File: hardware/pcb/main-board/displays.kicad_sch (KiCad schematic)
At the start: 1 part, among them J601 DISP_PCB x40 FPC

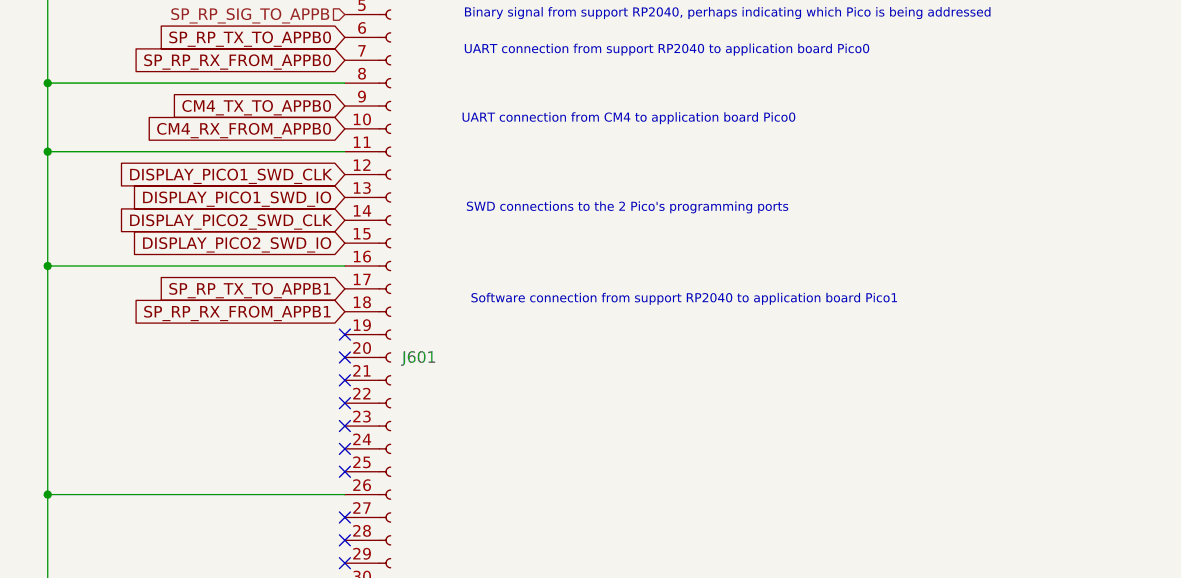
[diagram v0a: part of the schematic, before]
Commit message: tidy the keyboard comms
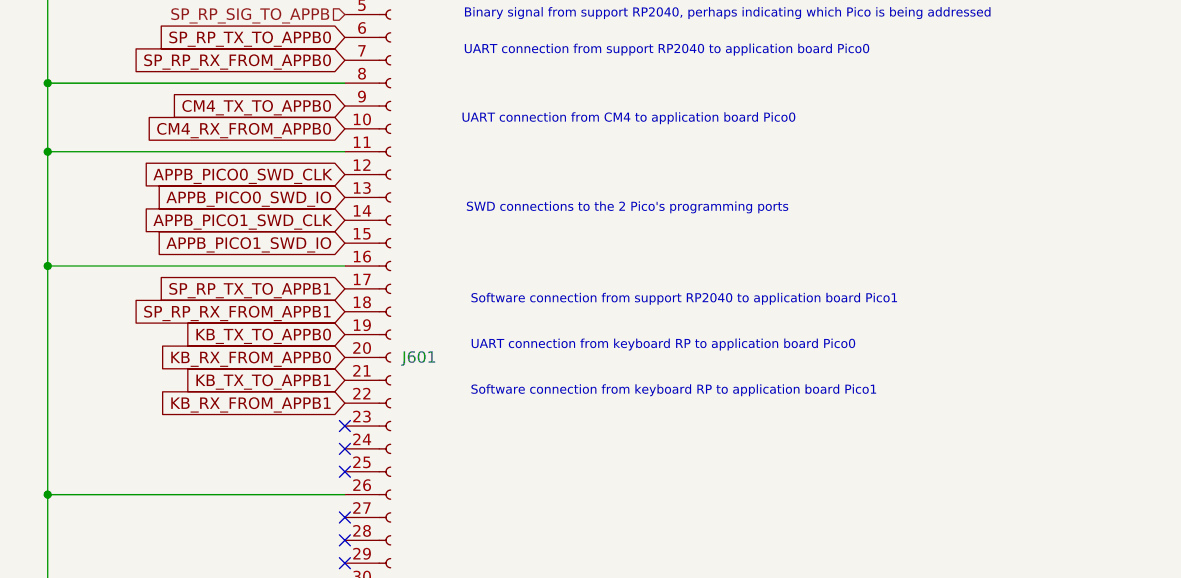
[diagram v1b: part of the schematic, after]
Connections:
- net KB_TX_TO_APPB0: now reaches J601.19 (Pin_19)
- net KB_RX_FROM_APPB0: now reaches J601.20 (Pin_20)
- net KB_TX_TO_APPB1: now reaches J601.21 (Pin_21)
- net KB_RX_FROM_APPB1: now reaches J601.22 (Pin_22)
- net DISPLAY_PICO1_SWD_CLK renamed APPB_PICO0_SWD_CLK
- net DISPLAY_PICO1_SWD_IO renamed APPB_PICO0_SWD_IO
- net DISPLAY_PICO2_SWD_CLK renamed APPB_PICO1_SWD_CLK
- net DISPLAY_PICO2_SWD_IO renamed APPB_PICO1_SWD_IO
- no-connect marks 15 -> 11
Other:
- note added: "Software connection from keyboard RP to application board Pico1"
- note added: "UART connection from keyboard RP to application board Pico0"
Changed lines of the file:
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@@
-	)
-	(no_connect
-		(at 58.42 68.58)
 	)
 	(no_connect
@@
 	)
 	(no_connect
-		(at 58.42 76.2)
-	)
-	(no_connect
-		(at 58.42 71.12)
-	)
-	(no_connect
 		(at 58.42 101.6)
 	)
@@
 		(at 58.42 99.06)
 	)
-	(no_connect
-		(at 58.42 73.66)
-	)
 	(wire
 		(pts
@@
 		)
 	)
+	(text "Software connection from keyboard RP to application board Pico1"
+		(exclude_from_sim no)
+		(at 72.39 74.93 0)
+		(effects
+			(font
+				(size 1 1)
+			)
+			(justify left)
+		)
+	)
 	(text "Software connection from support RP2040 to application board Pico1"
 		(exclude_from_sim no)
@@
 		)
 	)
+	(text "UART connection from keyboard RP to application board Pico0"
+		(exclude_from_sim no)
+		(at 72.39 69.85 0)
+		(effects
+			(font
+				(size 1 1)
+			)
+			(justify left)
+		)
+	)
 	(text "UART connection from CM4 to application board Pico0"
 		(exclude_from_sim no)
@@
 		)
 	)
-	(global_label "DISPLAY_PICO2_SWD_IO"
+	(global_label "APPB_PICO1_SWD_IO"
 		(shape input)
 		(at 58.42 58.42 180)
@@
 		)
 		(property "Intersheetrefs" "${INTERSHEET_REFS}"
-			(at 34.0756 58.42 0)
+			(at 36.7366 58.42 0)
 			(effects
 				(font
@@
 		)
 	)
-	(global_label "DISPLAY_PICO2_SWD_CLK"
+	(global_label "APPB_PICO1_SWD_CLK"
 		(shape input)
 		(at 58.42 55.88 180)
@@
 		)
 		(property "Intersheetrefs" "${INTERSHEET_REFS}"
-			(at 32.4428 55.88 0)
+			(at 35.1038 55.88 0)
 			(effects
 				(font
@@
 		)
 	)
-	(global_label "DISPLAY_PICO1_SWD_CLK"
+	(global_label "APPB_PICO0_SWD_CLK"
 		(shape input)
 		(at 58.42 50.8 180)
@@
 		)
 		(property "Intersheetrefs" "${INTERSHEET_REFS}"
-			(at 32.4428 50.8 0)
+			(at 35.1038 50.8 0)
 			(effects
 				(font
@@
 		)
 	)
-	(global_label "DISPLAY_PICO1_SWD_IO"
+	(global_label "KB_TX_TO_APPB1"
+		(shape input)
+		(at 58.42 73.66 180)
+		(fields_autoplaced yes)
+		(effects
+			(font
+				(size 1.27 1.27)
+			)
+			(justify right)
+		)
+		(property "Intersheetrefs" "${INTERSHEET_REFS}"
+			(at 40.0629 73.66 0)
+			(effects
+				(font
+					(size 1.27 1.27)
+				)
+				(justify right)
+				(hide yes)
+			)
+		)
+	)
+	(global_label "KB_RX_FROM_APPB0"
+		(shape input)
+		(at 58.42 71.12 180)
+		(fields_autoplaced yes)
+		(effects
+			(font
+				(size 1.27 1.27)
+			)
+			(justify right)
+		)
+		(property "Intersheetrefs" "${INTERSHEET_REFS}"
+			(at 36.9181 71.12 0)
+			(effects
+				(font
+					(size 1.27 1.27)
+				)
+				(justify right)
+				(hide yes)
+			)
+		)
+	)
+	(global_label "KB_TX_TO_APPB0"
+		(shape input)
+		(at 58.42 68.58 180)
+		(fields_autoplaced yes)
+		(effects
+			(font
+				(size 1.27 1.27)
+			)
+			(justify right)
+		)
+		(property "Intersheetrefs" "${INTERSHEET_REFS}"
+			(at 40.0629 68.58 0)
+			(effects
+				(font
+					(size 1.27 1.27)
+				)
+				(justify right)
+				(hide yes)
+			)
+		)
+	)
+	(global_label "APPB_PICO0_SWD_IO"
 		(shape input)
 		(at 58.42 53.34 180)
@@
 		)
 		(property "Intersheetrefs" "${INTERSHEET_REFS}"
-			(at 34.0756 53.34 0)
+			(at 36.7366 53.34 0)
 			(effects
 				(font
@@
 			(effects
 				(font
+					(size 1.27 1.27)
+				)
+				(justify right)
+				(hide yes)
+			)
+		)
+	)
+	(global_label "KB_RX_FROM_APPB1"
+		(shape input)
+		(at 58.42 76.2 180)
+		(fields_autoplaced yes)
+		(effects
+			(font
+				(size 1.27 1.27)
+			)
+			(justify right)
+		)
+		(property "Intersheetrefs" "${INTERSHEET_REFS}"
+			(at 36.9181 76.2 0)
+			(effects
+				(font
